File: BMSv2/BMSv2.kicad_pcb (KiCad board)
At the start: 2 copper layers, 126 parts, among them J1 Conn_01x05, J2 Conn_01x04_Socket, J3 Conn_01x02_Pin, J4 Conn_01x02_Pin, J5 Conn_01x03_Pin, Q1 AO3401A, Q10 MMBT3904, Q11 MMBT3904, Q12 MMBT3904, Q13 MMBT3904, Q14 Q_PNP_BEC, Q15 Q_PNP_BEC, Q16 Q_PNP_BEC, Q17 Q_PNP_BEC, Q2 MMBT3904, Q3 DMG2301L, Q4 MMBT3904, Q5 DMG2301L, Q6 MMBT3904, Q7 DMG2301L, Q8 MMBT3904, Q9 DMG2301L, SW1 SW_BOOT0, U1 STM32F405RGTx, U2 MCP2561-E-SN, U4 MP2332H, U5 AMS1117-3.3, Y1 Crystal_16MHz

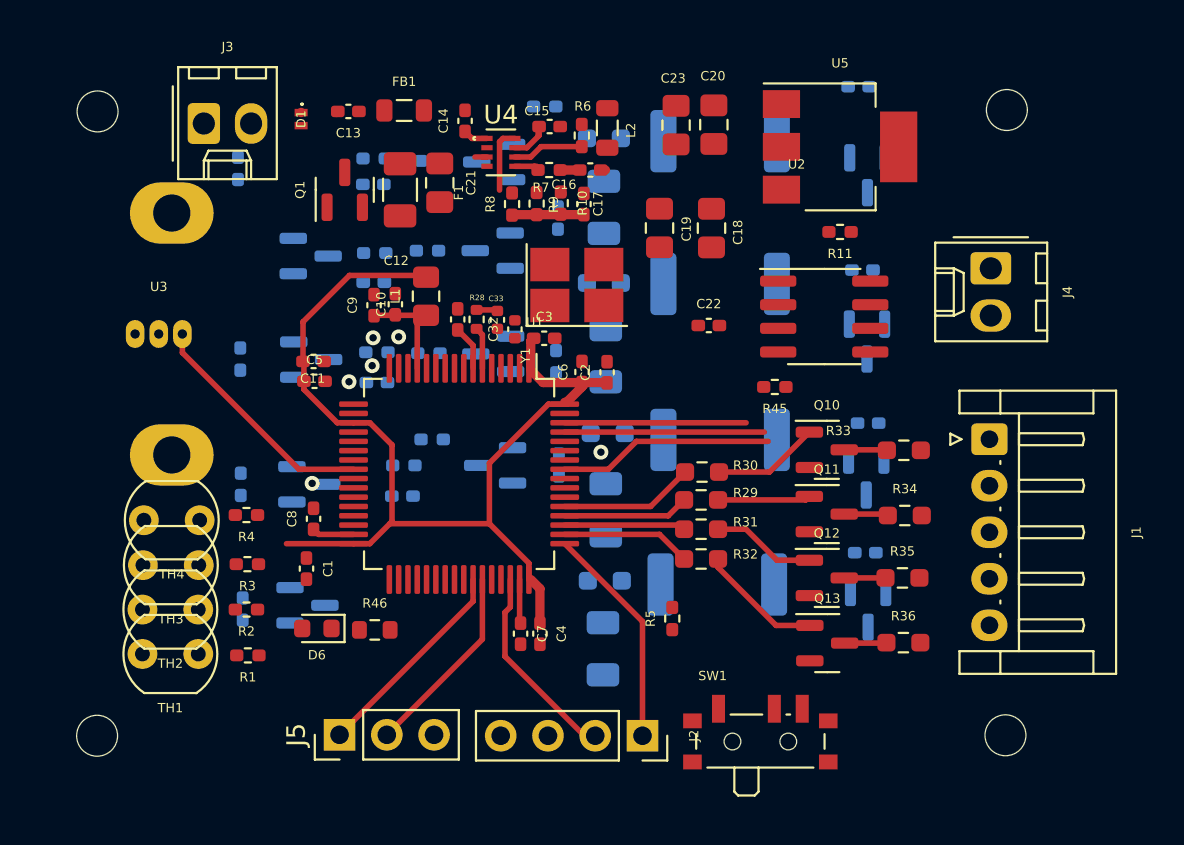
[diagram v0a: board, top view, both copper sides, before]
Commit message: Add files via upload
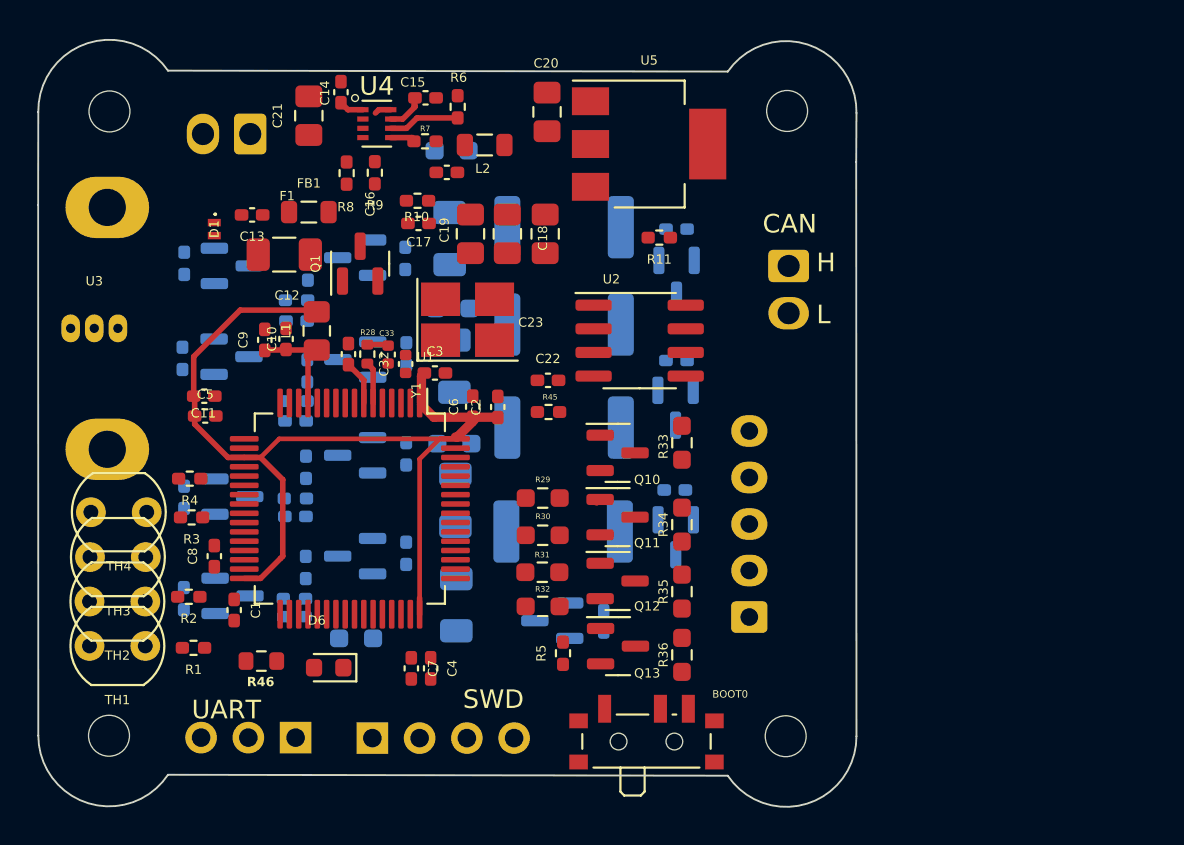
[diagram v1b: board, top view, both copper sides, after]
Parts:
- J1, J2, J3, J4, J5: moved to B.Cu
- moved Q17 17.0 mm to (97.1, 74.7), turned to 180 degrees
- moved J1 16.1 mm to (107.6, 74.5), turned to 90 degrees
- moved C27 14.5 mm to (99.8, 74.8), turned to 90 degrees
- moved J2 14.5 mm to (87.4, 81.1)
- moved R40 13.7 mm to (86.5, 75.7), turned to 180 degrees
- moved C24 12.4 mm to (103.7, 53.7)
- moved R45 12.2 mm to (96.9, 63.5)
- moved R34 12.0 mm to (104.0, 69.6), turned to 90 degrees
- moved R33 11.9 mm to (104.0, 65.2), turned to 90 degrees
- moved R36 11.9 mm to (104.0, 76.6), turned to 90 degrees
- moved R35 11.9 mm to (104.0, 73.2), turned to 90 degrees
- moved H1 11.8 mm to (109.7, 47.3)
- moved H2 11.8 mm to (109.6, 80.9)
- moved Q14 11.6 mm to (103.7, 56.3)
- moved Q10 11.2 mm to (100.6, 65.7)
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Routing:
- net Current: track 12.8 -> 0.00 mm
- net SWDCLK: track 12.1 -> 0.00 mm
- net CAN_STBY: track 11.6 -> 0.00 mm
- net UART_RX: track 11.3 -> 0.00 mm
- net SWDIO: track 10.9 -> 0.00 mm
- net CAN1_RX: track 10.7 -> 0.00 mm
- net UART_TX: track 10.5 -> 0.00 mm
- net CAN1_TX: track 9.75 -> 0.00 mm
- net CL4_DCH: track 7.24 -> 0.00 mm
- net CL1_DCH: track 6.96 -> 0.00 mm
- net CL3_DCH: track 6.77 -> 0.00 mm
- net CL2_DCH: track 6.51 -> 0.00 mm
- net Net-(Q13-B): track 6.68 -> 0.46 mm
- net Net-(Q10-B): track 5.74 -> 0.00 mm
- net Net-(Q12-B): track 5.60 -> 0.00 mm
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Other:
- board outline added: 44 x 41.2 mm
- board text added: "BOOT0"
- board text added: "CAN"
- board text added: "H"
- board text added: "L"
- board text added: "SWD"
- board text added: "UART"
